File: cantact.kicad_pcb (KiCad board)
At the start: 2 copper layers, 36 x 65.3 mm, 44 parts, among them J1 Cantact, P2 SWD, P4 USB_C_Plug_USB2.0, U1 STM32F042C6T6, U3 MCP2551-I/SN, U4 XC6220B331MR-G, X1 16 MHz

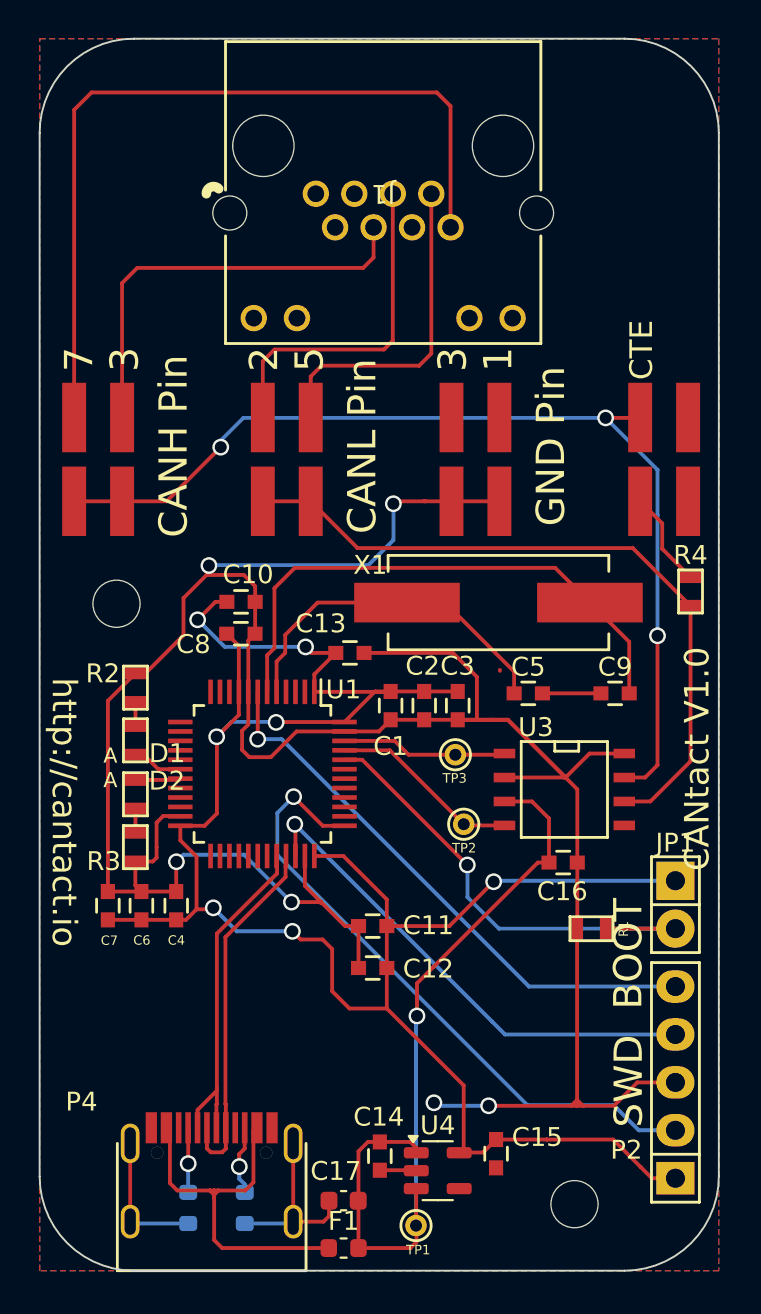
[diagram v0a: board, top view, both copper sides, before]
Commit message: refactor(hw): PCB routing
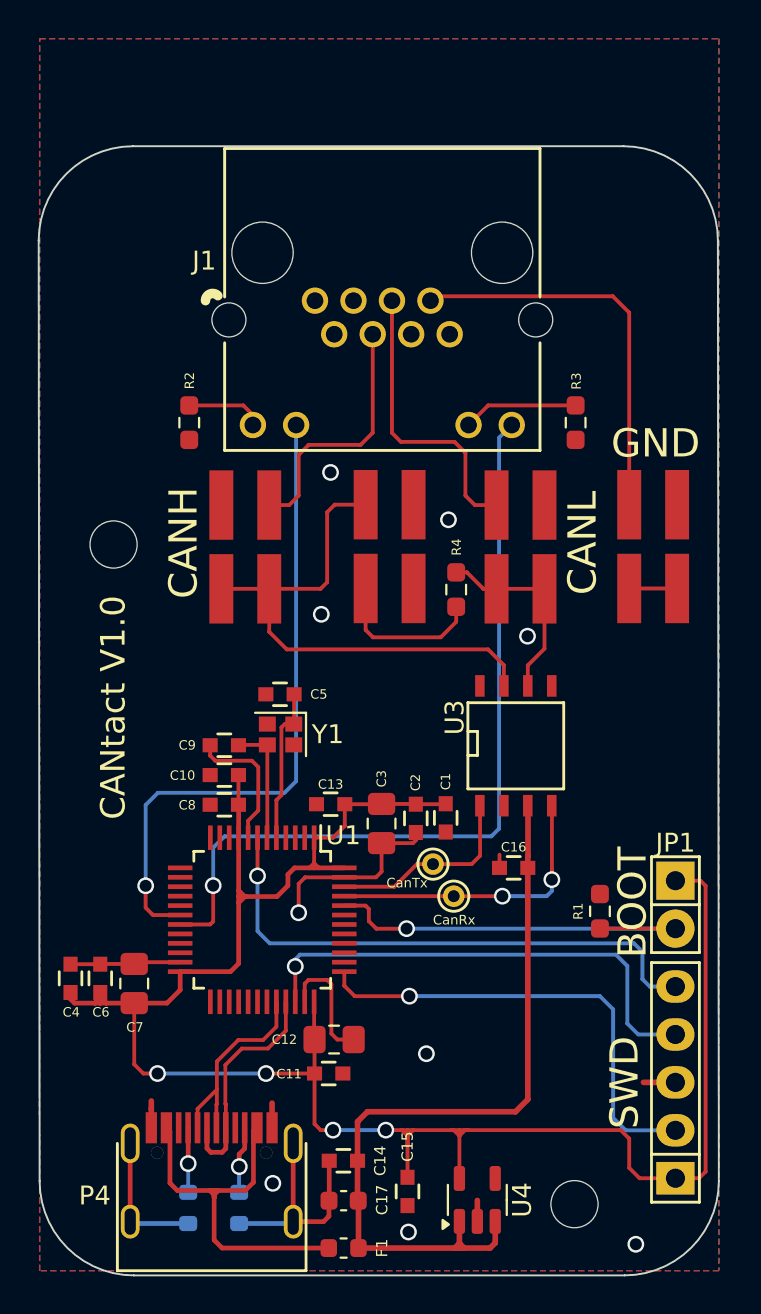
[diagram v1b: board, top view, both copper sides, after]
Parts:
- removed D1: LED-GREEN, SMD_Packages:SMD-0603
- removed D2: LED-RED, SMD_Packages:SMD-0603
- removed SYM: Symbol_OSHW-Logo_SilkScreen_07Jul2012, Symbols:Symbol_OSHW-Logo_SilkScreen
- removed TP1: TST, Connect:PINTST
- removed X1: 16 MHz, Crystals:Crystal_HC49-SD_SMD
- added Y1: 16 Mhz, Crystal:Crystal_SMD_2016-4Pin_2.0x1.6mm, F.Cu at (137.1, 123.4)
- C12, C3, C7: footprint Capacitors_SMD:C_0603 -> Capacitor_SMD:C_0805_2012Metric_Pad1.18x1.45mm_HandSolder
- R1, R2, R3, R4: footprint SMD_Packages:SMD-0603 -> Resistor_SMD:R_0603_1608Metric_Pad0.98x0.95mm_HandSolder
- moved R3 32.4 mm to (152.7, 106.8), turned to -90 degrees
- moved C9 20.9 mm to (134.1, 124.0)
- moved JP2 15.3 mm to (142.8, 113.4)
- moved R2 14.3 mm to (132.2, 106.9)
- moved JP4 13.2 mm to (149.8, 113.4)
- moved C5 13.2 mm to (137.0, 121.2), turned to 180 degrees
- moved R4 12.4 mm to (146.4, 115.7), turned to -90 degrees
- moved JP5 10.5 mm to (156.8, 113.4)
- moved C10 9.22 mm to (134.1, 125.5), turned to 180 degrees
- moved C8 9.11 mm to (134.1, 127.1), turned to 180 degrees
- moved JP3 9.08 mm to (135.2, 113.4)
- moved C11 8.16 mm to (139.6, 141.3), turned to 0 degrees
- moved C13 8.08 mm to (139.7, 127.1), turned to 180 degrees
- moved U1 7.73 mm to (136.1, 133.2)
- moved C3 7.44 mm to (142.4, 128.1)
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- renumbered TP2 to CanRx, TP3 to CanTx
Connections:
- J1 pad 10: unconnected-(J1-Pad10) -> Net-(J1-Pad10)
- J1 pad 11: unconnected-(J1-Pad11) -> /LED_GREEN
- J1 pad 12: unconnected-(J1-Pad12) -> Net-(J1-Pad12)
- J1 pad 4: /CANH2 -> /CANH1
- J1 pad 7: /CANL2 -> /GND1
- J1 pad 8: /CANH1 -> unconnected-(J1-Pad8)
- J1 pad 9: unconnected-(J1-Pad9) -> /LED_RED
- JP3 pad 2: /CANH1 -> /CANH2
- JP3 pad 4: /CANH2 -> /CANH1
- R2 pad 1: GND -> Net-(J1-Pad12)
- R2 pad 2: Net-(D1-K) -> GND
- R3 pad 1: GND -> Net-(J1-Pad10)
- R3 pad 2: Net-(D2-K) -> GND
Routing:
- net GND: track 175.0 -> 57.7 mm, vias 6 -> 9
- net /LED_RED: track 2.41 -> 43.0 mm, vias 0 -> 1
- net /LED_GREEN: track 2.70 -> 34.8 mm, vias 0 -> 1
- net /CANH1: track 43.4 -> 13.6 mm
- net Net-(JP4-Pin_1): track 37.6 -> 10.6 mm
- net Net-(JP2-Pin_2): track 53.7 -> 28.2 mm, vias 3 -> 0
- net Net-(U1-PF1-OSC_OUT): track 29.4 -> 6.47 mm
- net /CANH2: track 22.6 -> 0.00 mm
- net /GND1: track 0.00 -> 21.2 mm
- net /CANL2: track 17.5 -> 0.00 mm
- net Net-(U1-PF0-OSC_IN): track 20.3 -> 8.27 mm
- net /SWCLK: track 34.1 -> 24.8 mm
- net /D-: track 18.3 -> 11.7 mm
- net /D+: track 19.1 -> 12.7 mm
- net +3V3: track 115.4 -> 109.1 mm, vias 7 -> 4
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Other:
- board size 36 x 65.3 mm -> 36.1 x 59.9 mm
- board text added: "CANH"
- board text added: "CANL"
- board text added: "GND"
- board text removed: "2 5"
- board text removed: "3 1"
- board text removed: "7 3"
- board text removed: "A"
- board text removed: "CANH Pin"
- board text removed: "CANL Pin"
- board text removed: "CTE"
- board text removed: "GND Pin"
- board text removed: "http://cantact.io"
